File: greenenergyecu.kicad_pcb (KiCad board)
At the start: 2 copper layers, 17.5 x 11.5 mm, 1 part, among them M1 Module-knock-0.2

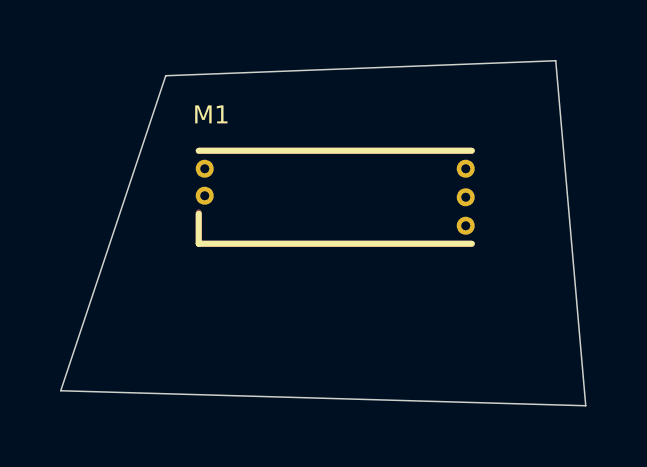
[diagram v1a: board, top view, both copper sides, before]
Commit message: err
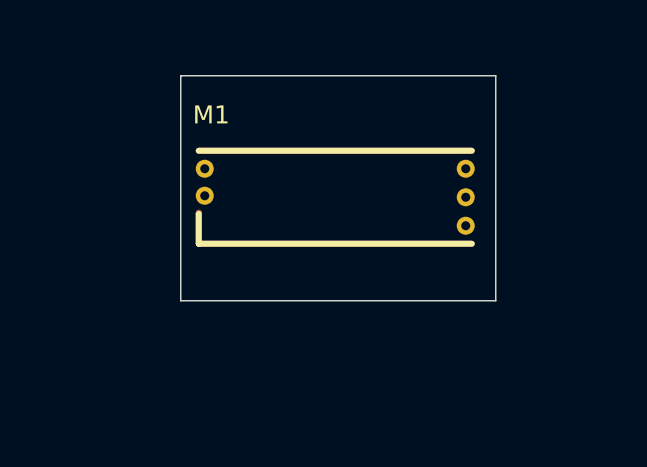
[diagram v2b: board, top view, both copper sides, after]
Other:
- board size 17.5 x 11.5 mm -> 10.5 x 7.5 mm
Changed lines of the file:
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@@
 		(pad_to_mask_clearance 0)
 		(allow_soldermask_bridges_in_footprints no)
-		(aux_axis_origin 119 64)
+		(aux_axis_origin 116 63.5)
+		(grid_origin 116 63.5)
 		(pcbplotparams
 			(layerselection 0x00010fc_ffffffff)
@@
 		)
 	)
-	(gr_poly
-		(pts
-			(xy 129.5 74.5) (xy 128.5 63) (xy 115.5 63.5) (xy 112 74)
-		)
+	(gr_rect
+		(start 116 63.5)
+		(end 126.5 71)
 		(stroke
 			(width 0.05)
-			(type solid)
+			(type default)
 		)
 		(fill none)

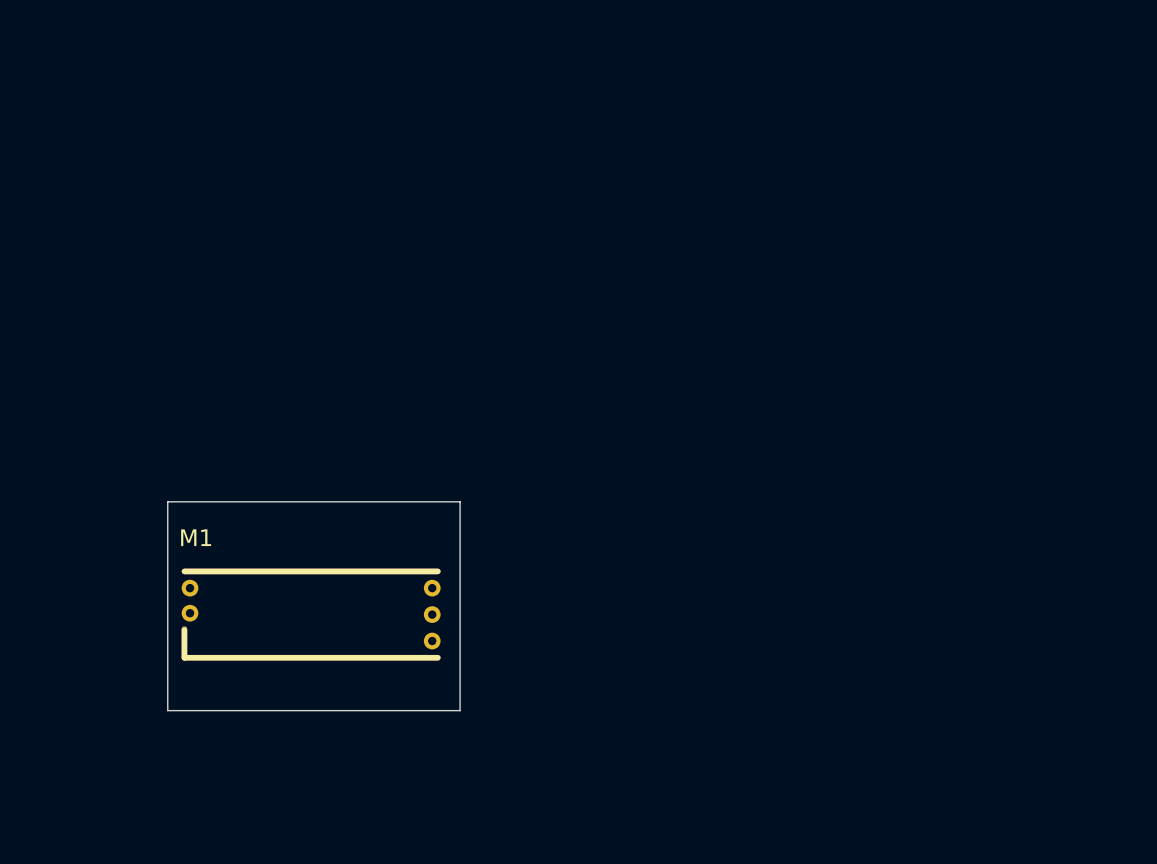
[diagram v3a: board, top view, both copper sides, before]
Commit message: ee
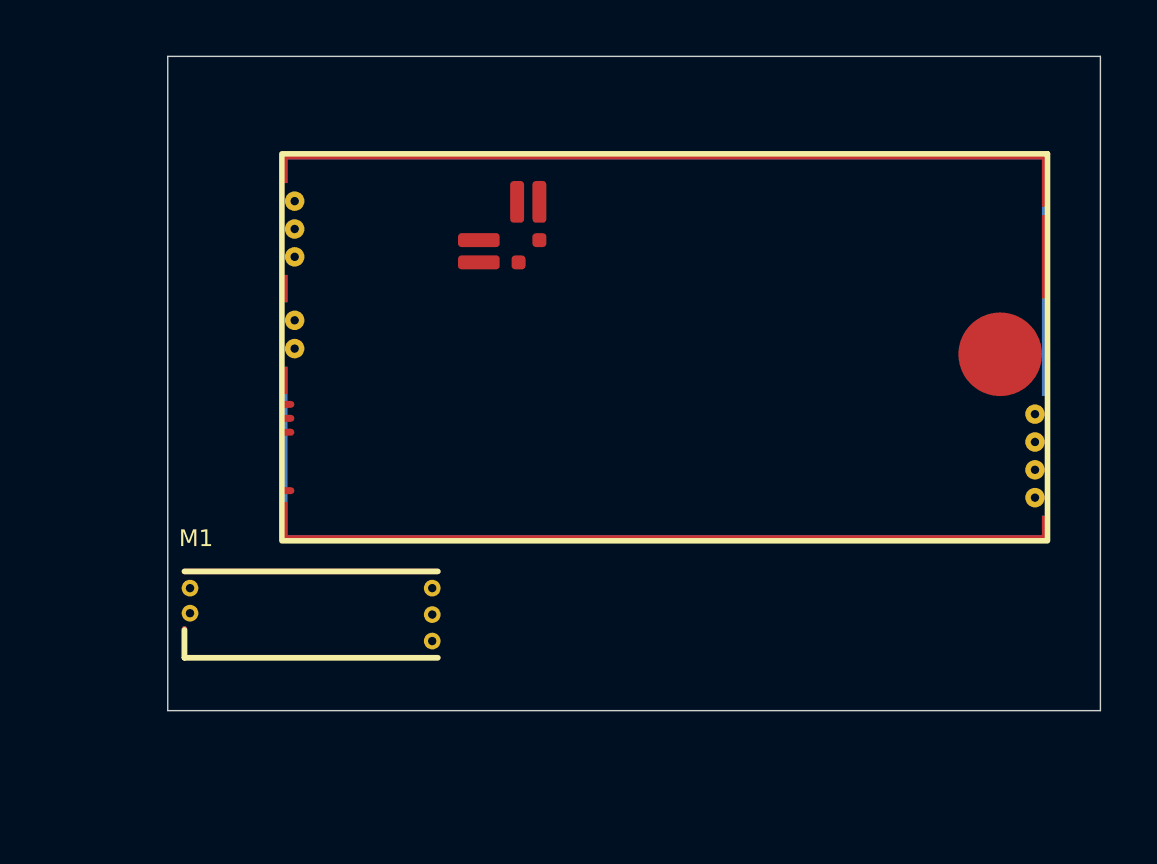
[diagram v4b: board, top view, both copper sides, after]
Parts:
- added REF**: M600, 0.5:wbo, F.Cu at (120.0, 65.0)
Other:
- board size 10.5 x 7.5 mm -> 33.5 x 23.5 mm
